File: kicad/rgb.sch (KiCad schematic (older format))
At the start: 14 parts, among them Q1 DMG9926USD, Q2 DMG9926USD, Q3 DMG9926USD, Q4 DMG9926USD, U1 ATTINY404-SSNR, U2 AP63205WU-7

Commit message: Cleaned up DC-DC
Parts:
- removed C4: 100 pF, symbol Device:C_Small
- removed L1: 2.2 uF, symbol Device:L_Small
- removed R2: 62 kΩ, symbol Device:R_Small_US
- added D1: LED, symbol Device:LED
- added L1: 4.7 uH, symbol Device:L
- R1: value 30.9 kΩ -> 1 kΩ
- renumbered C5 to C3
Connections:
- net labels added: +12V, +5V
- wire segments 30 -> 31
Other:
- note added: "DC-DC converter for MCU"
- moved on the sheet: C1, C2, C3, Q1A, Q1B, Q2A, Q2B, Q3A, Q3B, Q4A, Q4B, U1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

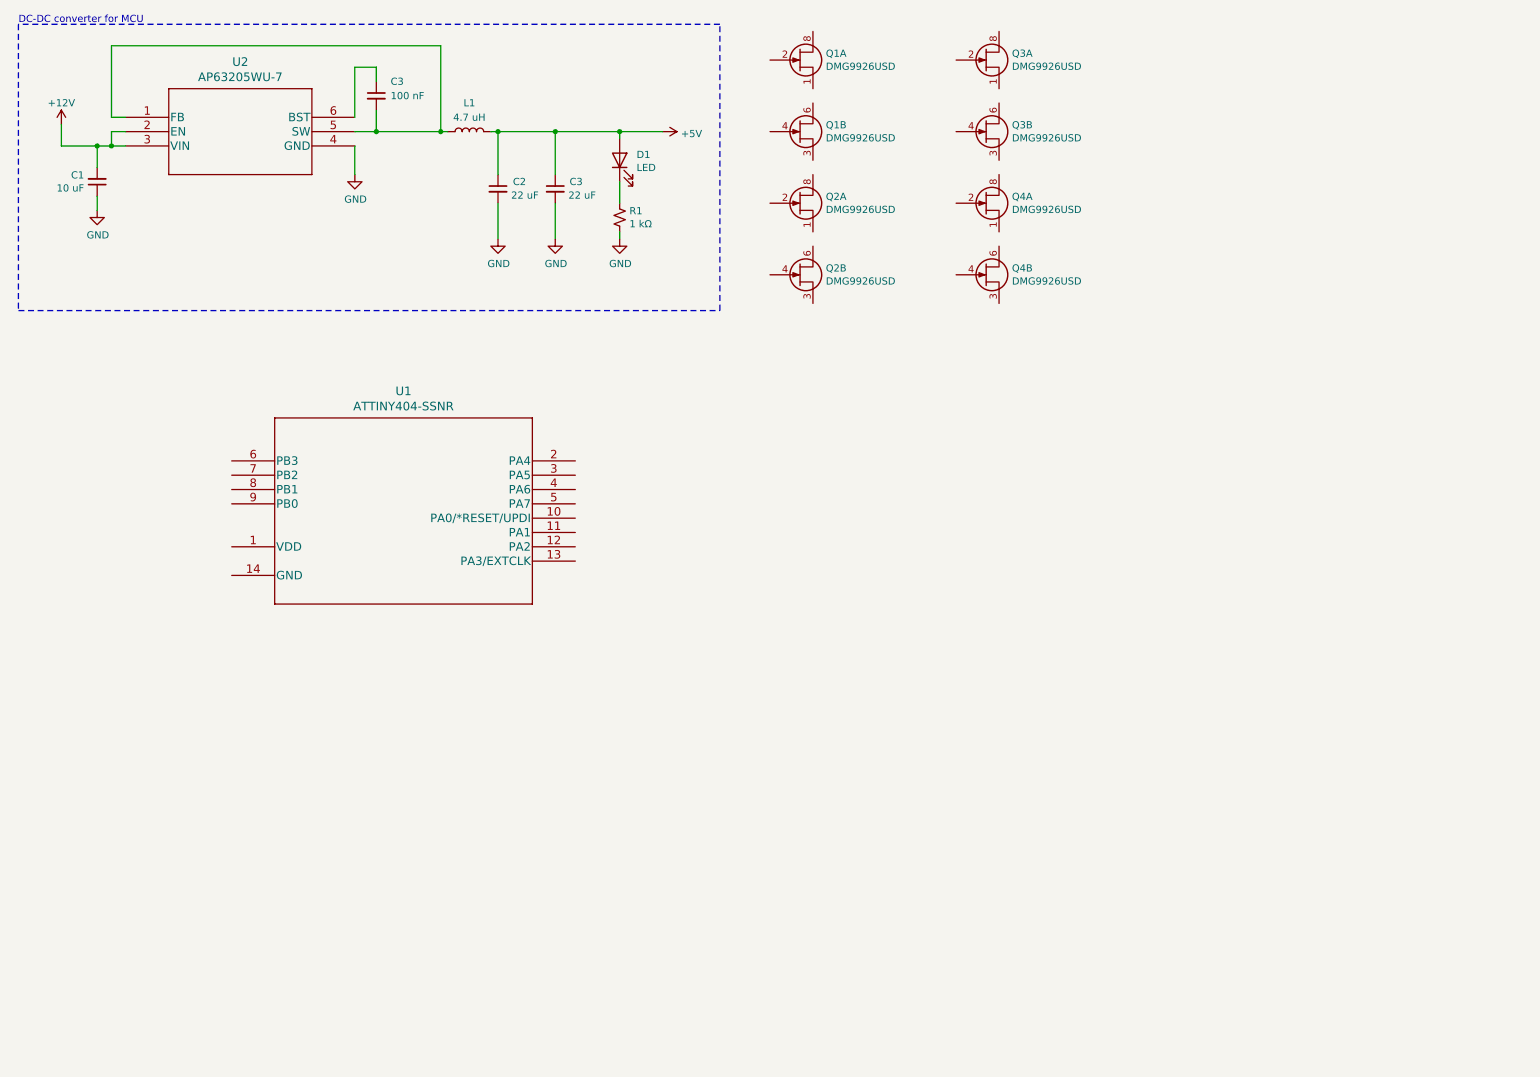
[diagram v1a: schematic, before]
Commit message: driver circuits
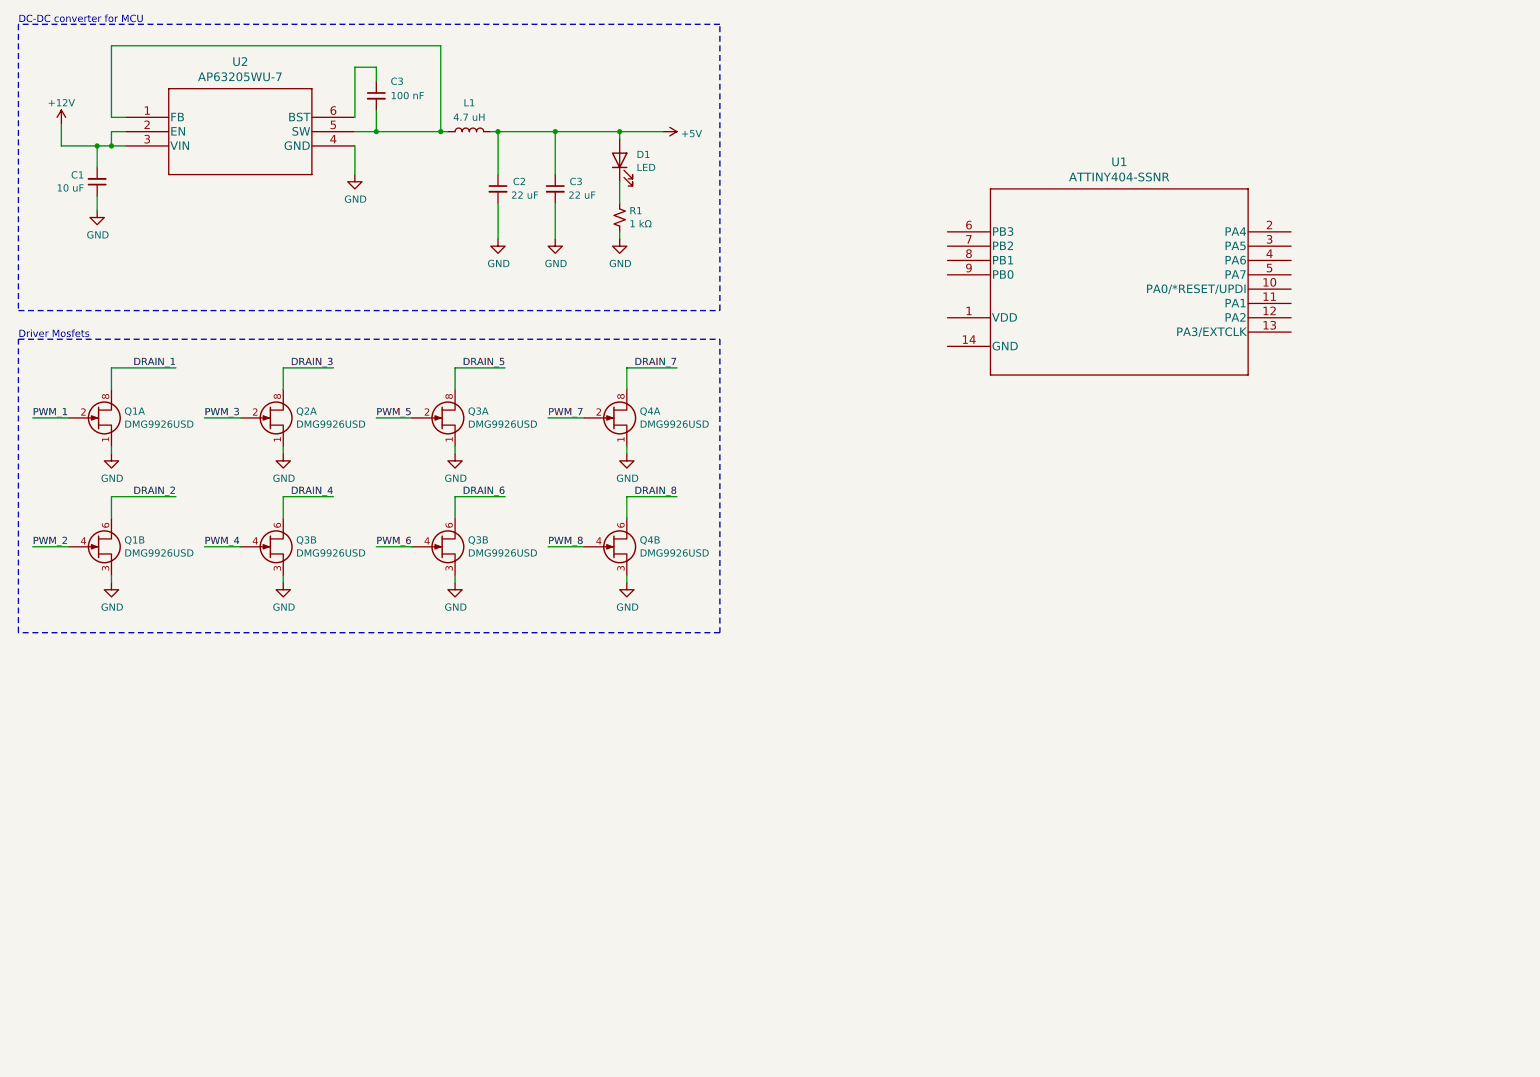
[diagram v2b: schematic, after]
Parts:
- removed unit 2 of Q2
- removed unit 2 of Q3
- added unit 2 of Q3 (x2)
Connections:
- net GND: now also Q1.1 (S1), Q1.3 (S2), Q2.1 (S1), Q3.1 (S1), Q4.1 (S1), Q4.3 (S2), Q3.3 (S2), Q3.3 (S2)
- net PWM_1: now reaches Q1.2 (G1)
- net DRAIN_1: now reaches Q1.8 (D1)
- net PWM_2: now reaches Q1.4 (G2)
- net DRAIN_2: now reaches Q1.6 (D2)
- net PWM_3: now reaches Q2.2 (G1)
- net DRAIN_3: now reaches Q2.8 (D1)
- net PWM_5: now reaches Q3.2 (G1)
- net DRAIN_5: now reaches Q3.8 (D1)
- net PWM_7: now reaches Q4.2 (G1)
- net DRAIN_7: now reaches Q4.8 (D1)
- net PWM_8: now reaches Q4.4 (G2)
- net DRAIN_8: now reaches Q4.6 (D2)
- new net DRAIN_4: Q3.6 (D2)
- new net DRAIN_6: Q3.6 (D2)
- new net PWM_4: Q3.4 (G2)
- new net PWM_6: Q3.4 (G2)
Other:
- note added: "Driver Mosfets"
- moved on the sheet: Q1A, U1

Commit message: ATTINY216
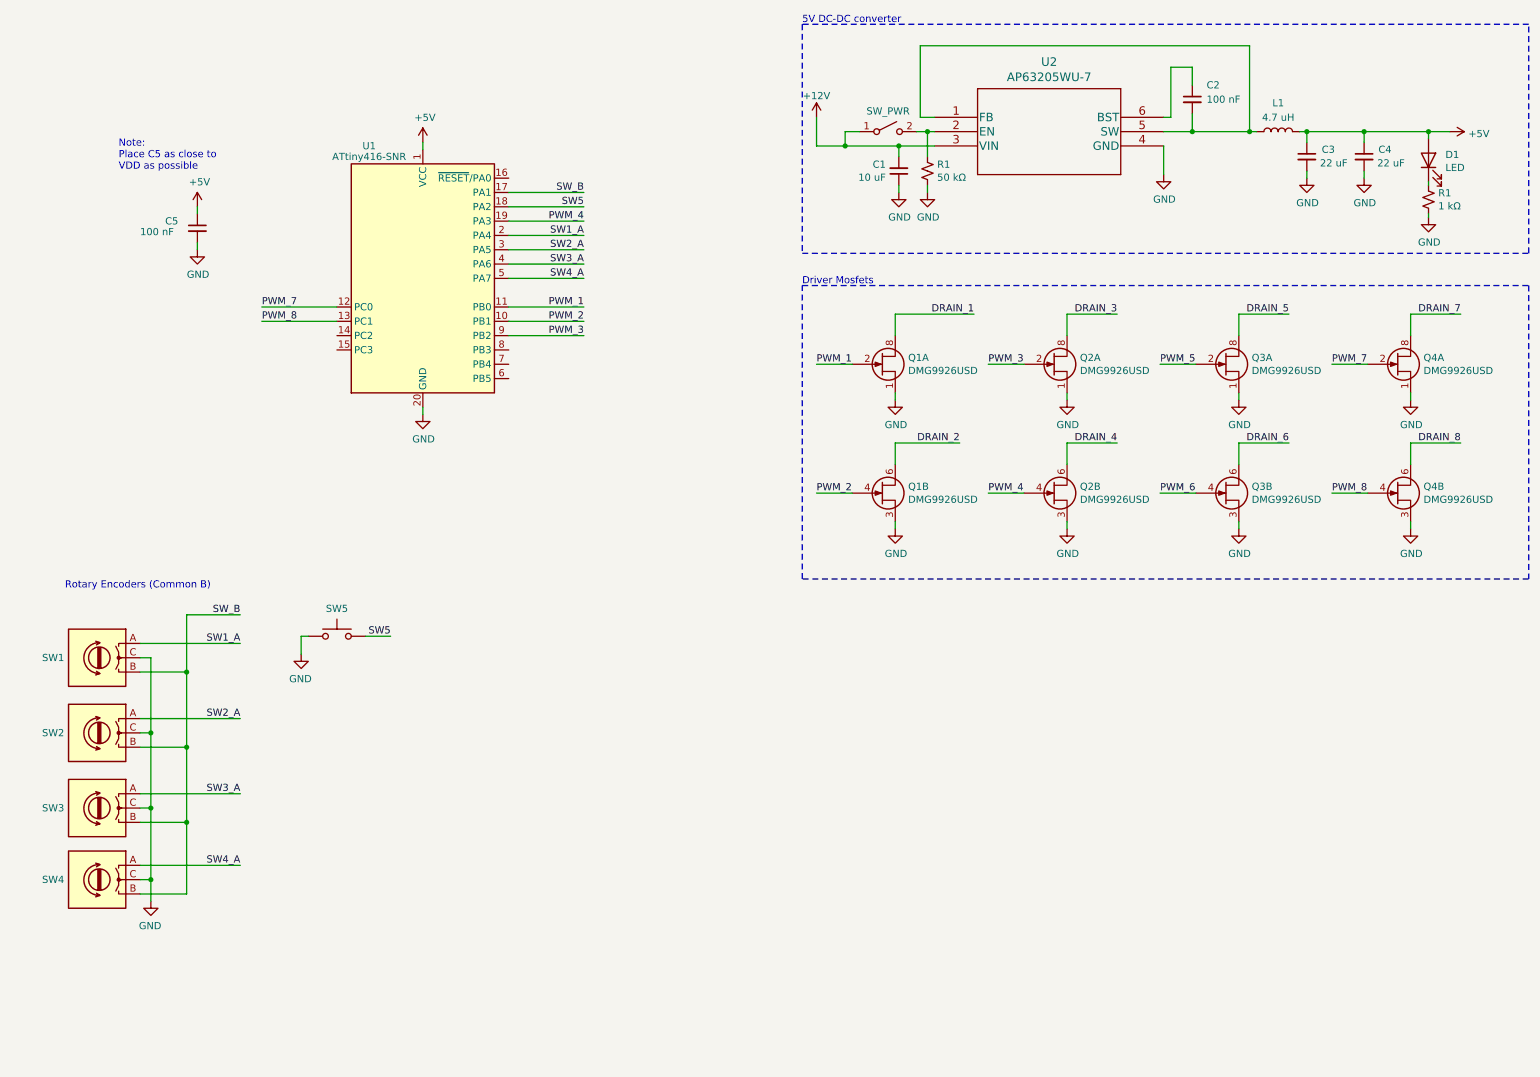
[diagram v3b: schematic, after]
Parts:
- removed U1: ATTINY404-SSNR, rgb_footprints:ATTINY404-SSNR, symbol ATTINY404-SSNR:ATTINY404-SSNR
- added C5: 100 nF, symbol Device:C_Small
- added R1: 50 kΩ, symbol Device:R_Small_US
- added SW1, SW2, SW3, SW4: Rotary_Encoder, symbol Device:Rotary_Encoder
- added SW5: SW_Push, symbol Switch:SW_Push
- added SW_PWR: 1825232-1, symbol Switch:SW_SPST
- added U1: ATtiny416-SNR, Package_SO:SOIC-20W_7.5x12.8mm_P1.27mm, symbol MCU_Microchip_ATtiny:ATtiny416-S
- renumbered C3 to C2, C2 to C3, C3 to C4, Q3 to Q2
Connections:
- net +12V: now also SW_PWR.1 (A); no longer U2.2 (EN)
- net +5V: now also C5.1, U1.1 (VCC)
- net GND: now also C5.2, R1.2, SW1.C, SW2.C, SW3.C, SW4.C, SW5.1, U1.20 (GND)
- net PWM_1: now also U1.11 (PB0)
- net PWM_2: now also U1.10 (PB1)
- net PWM_3: now also U1.9 (PB2)
- net PWM_4: now also U1.19 (PA3)
- net PWM_7: now also U1.12 (PC0)
- net PWM_8: now also U1.13 (PC1)
- new net: R1.1, SW_PWR.2 (B), U2.2 (EN)
- new net SW1_A: SW1.A, U1.2 (PA4)
- new net SW2_A: SW2.A, U1.3 (PA5)
- new net SW3_A: SW3.A, U1.4 (PA6)
- new net SW4_A: SW4.A, U1.5 (PA7)
- new net SW5: SW5.2, U1.18 (PA2)
- new net SW_B: SW1.B, SW2.B, SW3.B, SW4.B, U1.17 (PA1)
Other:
- note added: "5V DC-DC converter"
- note added: "Note:\nPlace C5 as close to\nVDD as possible"
- note added: "Rotary Encoders (Common B)"
- note removed: "DC-DC converter for MCU"
- moved on the sheet: C1, C2, C3, C4, D1, L1, Q1A, Q1B, Q2A, Q2B, Q3A, Q3B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

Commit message: Schematics work
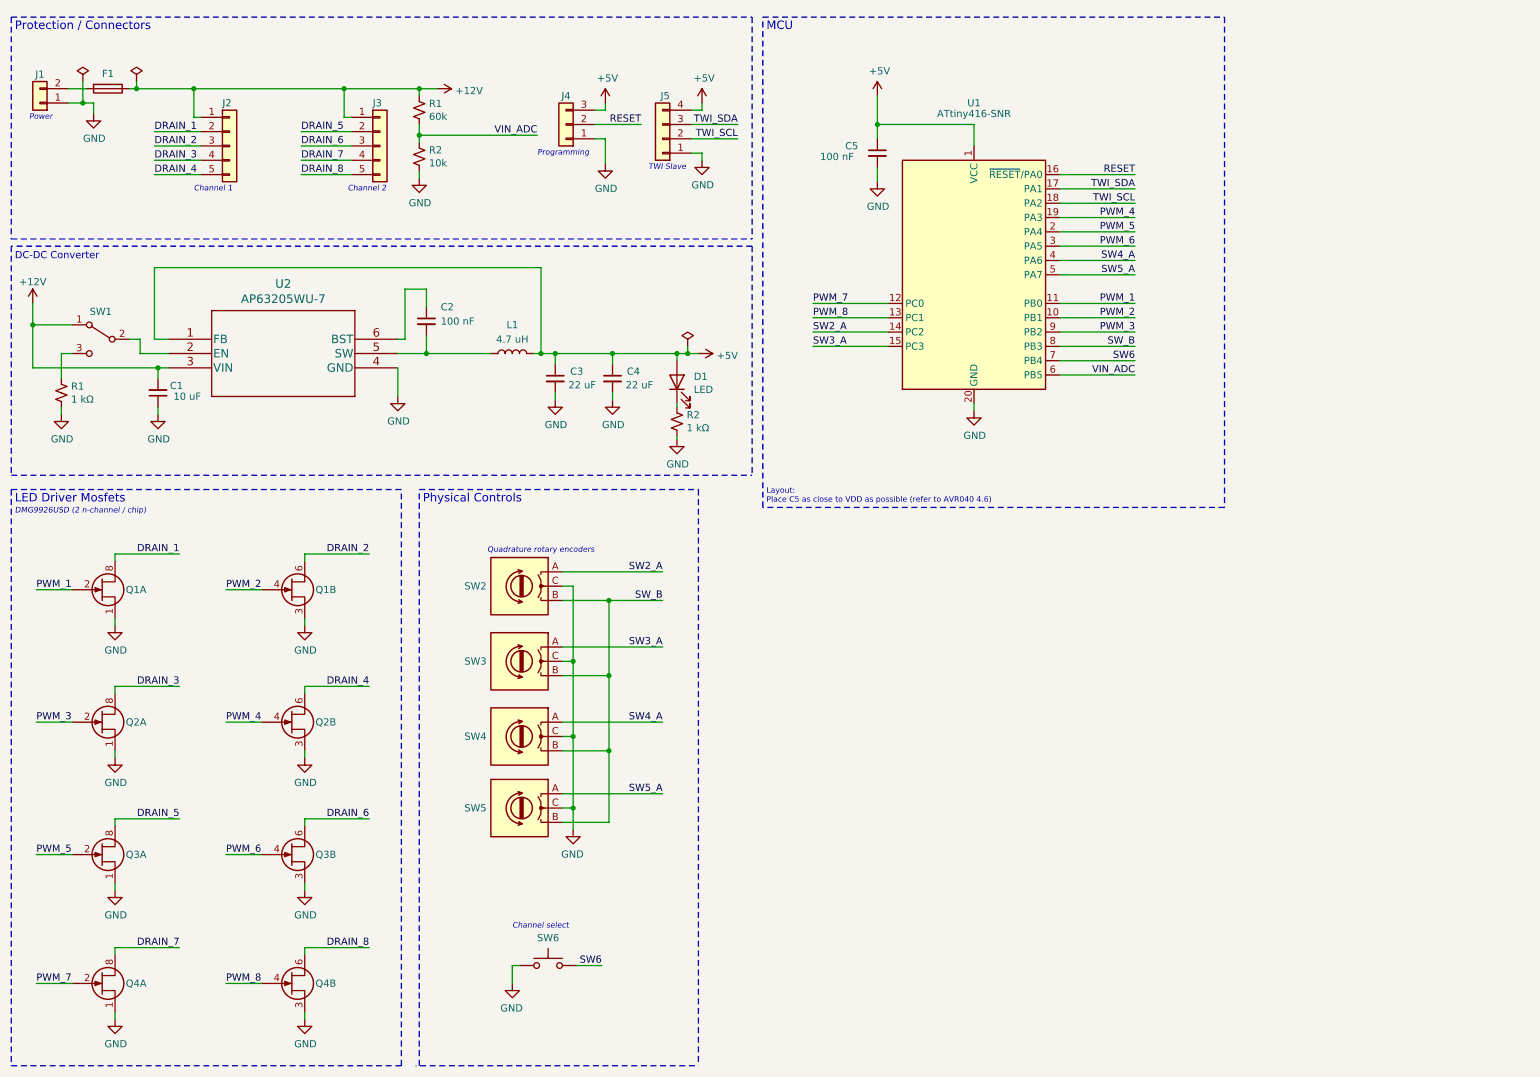
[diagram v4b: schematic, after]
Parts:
- removed unit 1 of Q3
- removed unit 1 of Q4
- removed R1: 50 kΩ, symbol Device:R_Small_US
- removed SW_PWR: 1825232-1, symbol Switch:SW_SPST
- added F1: 0685H9200-01, Fuse:Fuse_1206_3216Metric_Pad1.42x1.75mm_HandSolder, symbol Device:Fuse
- added J1: 1935776, symbol Connector_Generic:Conn_01x02
- added J2, J3: Conn_01x05, symbol Connector_Generic:Conn_01x05
- added J4: Conn_01x04, symbol Connector_Generic:Conn_01x03
- added J5: Conn_01x02, symbol Connector_Generic:Conn_01x04
- added unit 2 of Q1
- added unit 2 of Q2
- added R1: 1 kΩ, symbol Device:R_Small_US
- added R1: 60k, symbol Device:R_Small_US
- added R2: 10k, symbol Device:R_Small_US
- added SW1: 1825232-1, rgb_footprints:Switch_Slide_1825232-1, symbol Switch:SW_SPDT
- Q1, Q3, Q4: footprint Package_SO:SO-8_3.9x4.9mm_P1.27mm -> rgb_footprints:DMG9926USD_Handsolder
- Q2: renamed from Q1; footprint Package_SO:SO-8_3.9x4.9mm_P1.27mm -> rgb_footprints:DMG9926USD_Handsolder
- Q3, Q4: renamed from Q2; footprint Package_SO:SO-8_3.9x4.9mm_P1.27mm -> rgb_footprints:DMG9926USD_Handsolder
- U1: footprint Package_SO:SOIC-20W_7.5x12.8mm_P1.27mm -> rgb_footprints:ATTINY416-SNR
- U2: footprint SOIC_05WU-7_DIO -> rgb_footprints:AP63205WU-7
- renumbered R1 to R2, SW1 to SW2, SW2 to SW3, SW3 to SW4, SW4 to SW5, SW5 to SW6
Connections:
- net +12V: now also F1.1, J2.1 (Pin_1), J3.1 (Pin_1), R1.1, SW1.1 (A)
- net +5V: now also U2.1 (FB), J4.3 (Pin_3), J5.4 (Pin_4)
- net DRAIN_1: now also J2.2 (Pin_2)
- net DRAIN_2: now also J2.3 (Pin_3), Q1.6 (D2); no longer Q2.6 (D2)
- net DRAIN_3: now also Q2.8 (D1), J2.4 (Pin_4); no longer Q3.8 (D1)
- net DRAIN_4: now also J2.5 (Pin_5), Q2.6 (D2); no longer Q4.6 (D2)
- net DRAIN_5: now also Q3.8 (D1), J3.2 (Pin_2)
- net DRAIN_6: now also J3.3 (Pin_3)
- net DRAIN_7: now also Q4.8 (D1), J3.4 (Pin_4)
- net DRAIN_8: now also J3.5 (Pin_5)
- net GND: now also Q2.1 (S1), Q4.1 (S1), J1.1 (Pin_1), J4.1 (Pin_1), J5.1 (Pin_1), Q1.3 (S2), Q2.3 (S2), R1.2, R2.2; no longer Q2.3 (S2), Q4.3 (S2)
- net PWM_2: now also Q1.4 (G2); no longer Q2.4 (G2)
- net PWM_3: now also Q2.2 (G1); no longer Q3.2 (G1)
- net PWM_4: now also Q2.4 (G2); no longer Q4.4 (G2)
- net PWM_5: now also Q3.2 (G1), U1.2 (PA4)
- net PWM_6: now also U1.3 (PA5)
- net PWM_7: now also Q4.2 (G1)
- net SW2_A: now also SW2.A, U1.14 (PC2); no longer SW3.A, U1.3 (PA5)
- net SW3_A: now also SW3.A, U1.15 (PC3); no longer SW4.A, U1.4 (PA6)
- net SW4_A: now also SW4.A, U1.4 (PA6); no longer SW5.A, U1.5 (PA7)
- net SW_B: now also U1.8 (PB3); no longer U1.17 (PA1)
- net at C2.2, L1.1, U2.5 (SW): no longer U2.1 (FB)
- net at U2.2 (EN): now also SW1.2 (B)
- net RESET: now reaches U1.16 (~RESET~/PA0)
- net RESET: now also J4.2 (Pin_2)
- net VIN_ADC: now reaches U1.6 (PB5)
- net VIN_ADC: now also R1.2, R2.1
- net SW6: now reaches U1.7 (PB4)
- net SW6: now also SW6.2
- removed net SW1_A: SW2.A, U1.2 (PA4)
- net SW5 renamed TWI_SCL
- net TWI_SCL: now also J5.2 (Pin_2); no longer SW6.2
- new net: R1.1, SW1.3 (C)
- new net: F1.2, J1.2 (Pin_2)
- new net SW5_A: SW5.A, U1.5 (PA7)
- new net TWI_SDA: J5.3 (Pin_3), U1.17 (PA1)
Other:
- note added: "Channel 1"
- note added: "Channel 2\n"
- note added: "Channel select\n"
- note added: "DC-DC Converter"
- note added: "DMG9926USD (2 n-channel / chip)"
- note added: "LED Driver Mosfets"
- note added: "Layout:\nPlace C5 as close to VDD as possible (refer to AVR040 4.6)"
- note added: "MCU"
- note added: "Physical Controls"
- note added: "Power"
- note added: "Programming"
- note added: "Protection / Connectors\n"
- note added: "Quadrature rotary encoders"
- note added: "TWI Slave"
- note removed: "5V DC-DC converter"
- note removed: "Driver Mosfets"
- note removed: "Note:\nPlace C5 as close to\nVDD as possible"
- note removed: "Rotary Encoders (Common B)"
- moved on the sheet: C1, C2, C3, C4, C5, D1, L1, Q1A, Q3A, R2, SW2, SW3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
